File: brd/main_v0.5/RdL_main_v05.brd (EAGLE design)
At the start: 56.7 x 30.2 mm, 50 parts, among them J1 Test, J10 VCC, J11 LEDS1, J12 LEDS1, J13 LEDS1, J14 LEDS1, J3 GND, J4 GND, J5 GND, J6 GND, J7 VCC, J8 VCC, J9 VCC, U1 MPU-6000QFN-24

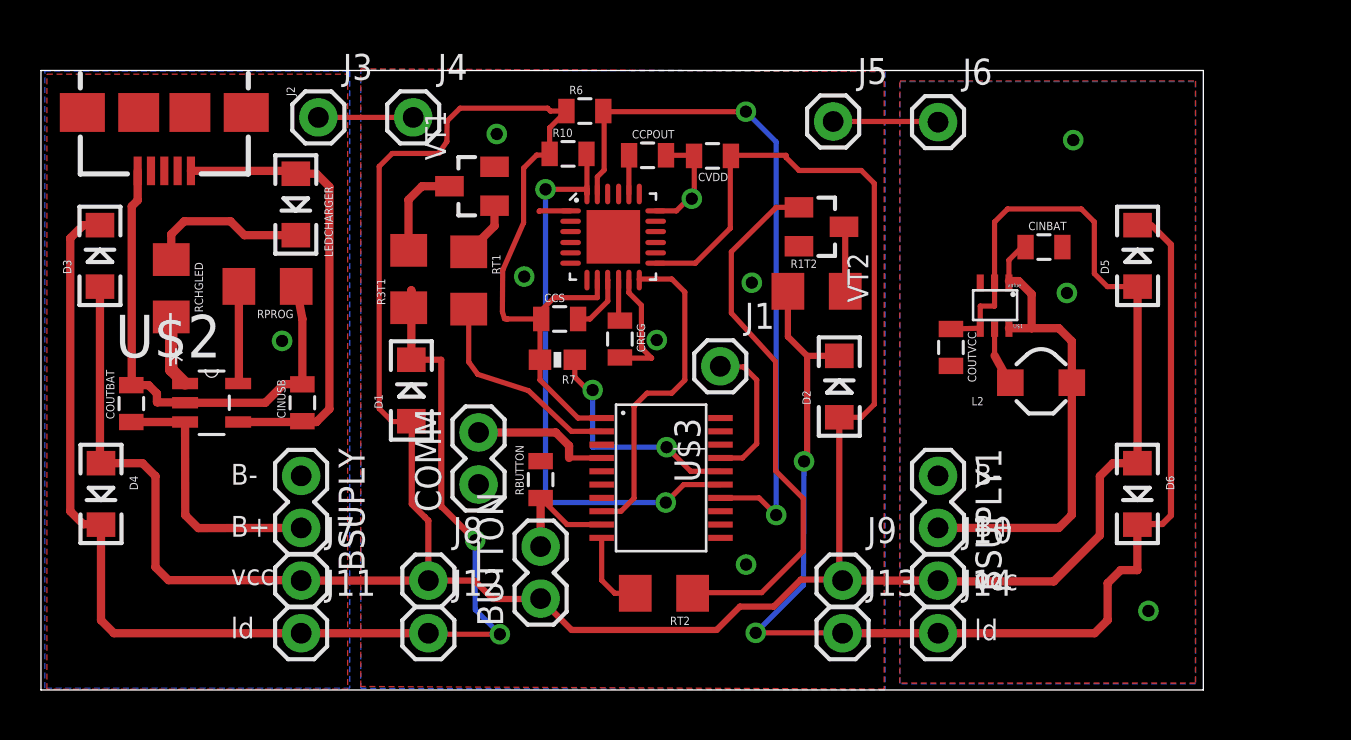
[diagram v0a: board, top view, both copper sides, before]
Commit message: RdL version 5 ready to print
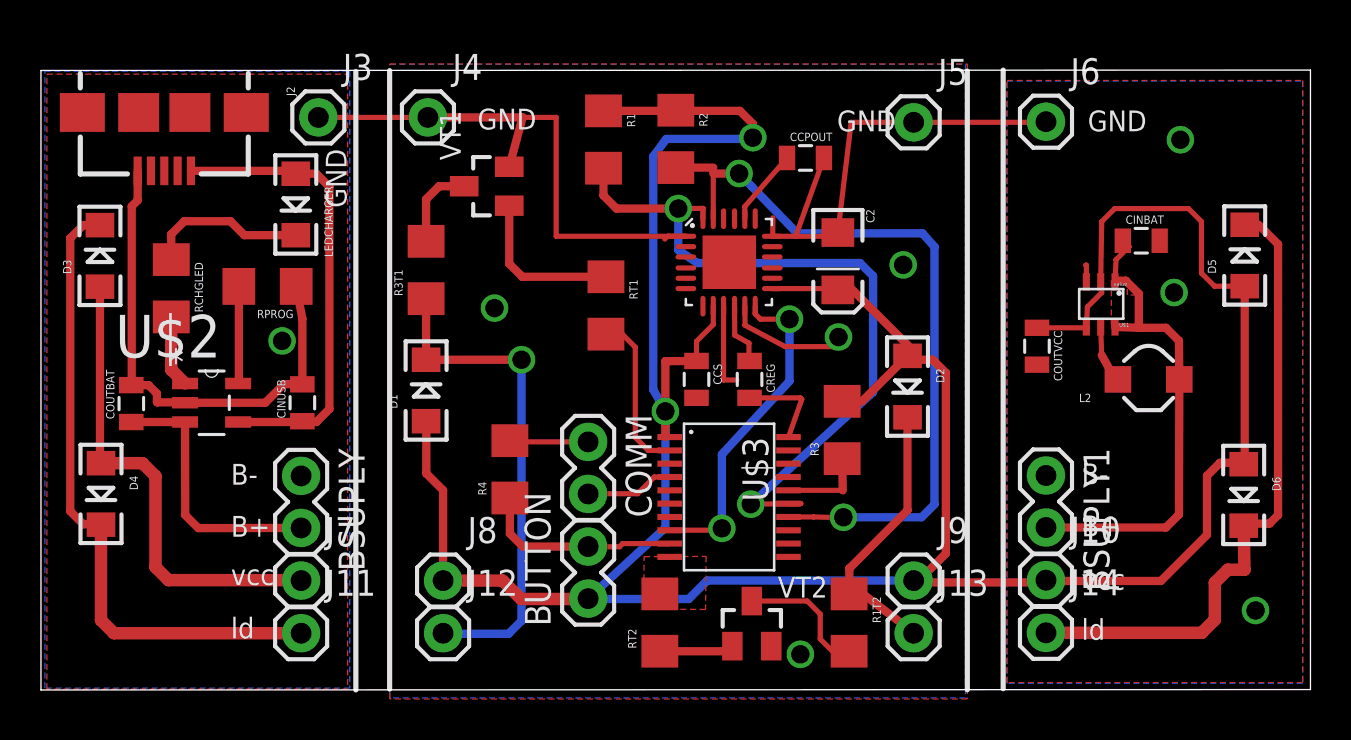
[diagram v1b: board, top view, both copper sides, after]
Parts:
- removed CVDD: 100nF, SparkFun-Capacitors:0805
- removed J1: Test, SparkFun-Connectors:1X01
- removed R10, R6, RBUTTON: 10k, SparkFun-Resistors:0805
- removed R7: 47K, SparkFun-Resistors:0603-RES
- added C2: 4.7uF, SparkFun-Capacitors:EIA3216
- added R1, R2: 4.7k, SparkFun-Resistors:1206
- added R3: 47k, SparkFun-Resistors:1206
- added R4: 10k, SparkFun-Resistors:1206
- CREG: value 100nF -> 0.1uF
- moved VT2 19.7 mm to (34.7, 3.24), turned to 0 degrees
- moved R1T2 16.2 mm to (39.5, 3.29), turned to 270 degrees
- moved CCPOUT 7.71 mm to (37.3, 26.0)
- moved CCS 7.30 mm to (32.0, 15.2), turned to 270 degrees
- moved RT1 6.81 mm to (27.6, 18.8)
- moved CREG 6.63 mm to (34.6, 15.2)
- moved U1 5.79 mm to (33.6, 20.9)
- moved COMM 5.74 mm to (26.7, 12.1), turned to 270 degrees
- moved BSUPLY1 5.27 mm to (49.1, 10.5)
- moved J10 5.27 mm to (49.1, 5.36)
- moved J14 5.27 mm to (49.1, 2.79)
- moved J6 5.27 mm to (49.1, 27.7)
- moved L2 5.25 mm to (54.1, 15.2)
- moved D5 5.23 mm to (58.8, 21.2)
- moved D6 5.19 mm to (58.7, 9.52)
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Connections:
- removed net N$4: J1.1, U$3.17
- net GND: now also C2.C, R4.2; no longer CVDD.2, RBUTTON.2
- net N$1: now also R4.1; no longer RBUTTON.1
- net N$12: now also R3.1; no longer R7.1
- net N$20: now also R1.2; no longer R10.2
- net N$22: now also R2.2; no longer R6.2
- net VCC: now also C2.A, R1.1, R2.1, R3.2; no longer CVDD.1, R10.1, R6.1, R7.2
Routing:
- net GND: track 50.2 -> 95.8 mm, vias 10 -> 8
- net N$9: track 26.5 -> 3.64 mm
- net N$13: track 59.9 -> 45.3 mm, vias 2 -> 0
- net VCC: track 189.3 -> 174.7 mm, vias 0 -> 2
- net N$20: track 28.4 -> 35.8 mm
- net N$12: track 11.5 -> 4.20 mm, vias 2 -> 0
- net N$4: track 7.23 -> 0.00 mm
- net N$14: track 61.6 -> 56.0 mm, vias 2 -> 1
- net N$8: track 2.77 -> 7.82 mm
- net N$1: track 5.89 -> 9.87 mm
- net N$11: track 3.97 -> 0.48 mm
- net N$6: track 3.21 -> 6.51 mm
- net N$15: track 6.87 -> 4.32 mm
- net N$10: track 10.3 -> 8.04 mm
- net N$22: track 34.5 -> 36.7 mm
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- added copper zone on layer 1, net N$11
- added copper zone on layer 1, net VOUTBATT
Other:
- board size 56.7 x 30.2 mm -> 62 x 30.3 mm
- board text added: "GND"
